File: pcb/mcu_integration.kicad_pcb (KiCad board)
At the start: 4 copper layers, 100 x 100 mm, 104 parts, among them IC1 TL7660IDGKR, IC10 AD844_OPAMP_MEL, IC2 TL081IDT, IC3 FOD814_OPTO_NOSHD, IC4 UA78M33CDCYG3, IC5 FOD814_OPTO_MEL, IC6 AD844_OPAMP_AL, IC7 FOD814_OPTO_AL, IC8 AD844_OPAMP_NOSHD, J1 Micro_SD_Card, J2 M22-6003005, J3 Conn_01x06, U1 STM32F103RBTx, U2 REF192_NOSHD, U3 REF192_AL, U4 REF192_MEL, U5 TPS2069CDBVR_MOSFET, Y1 ECS-80-18-5PX-GM-TR

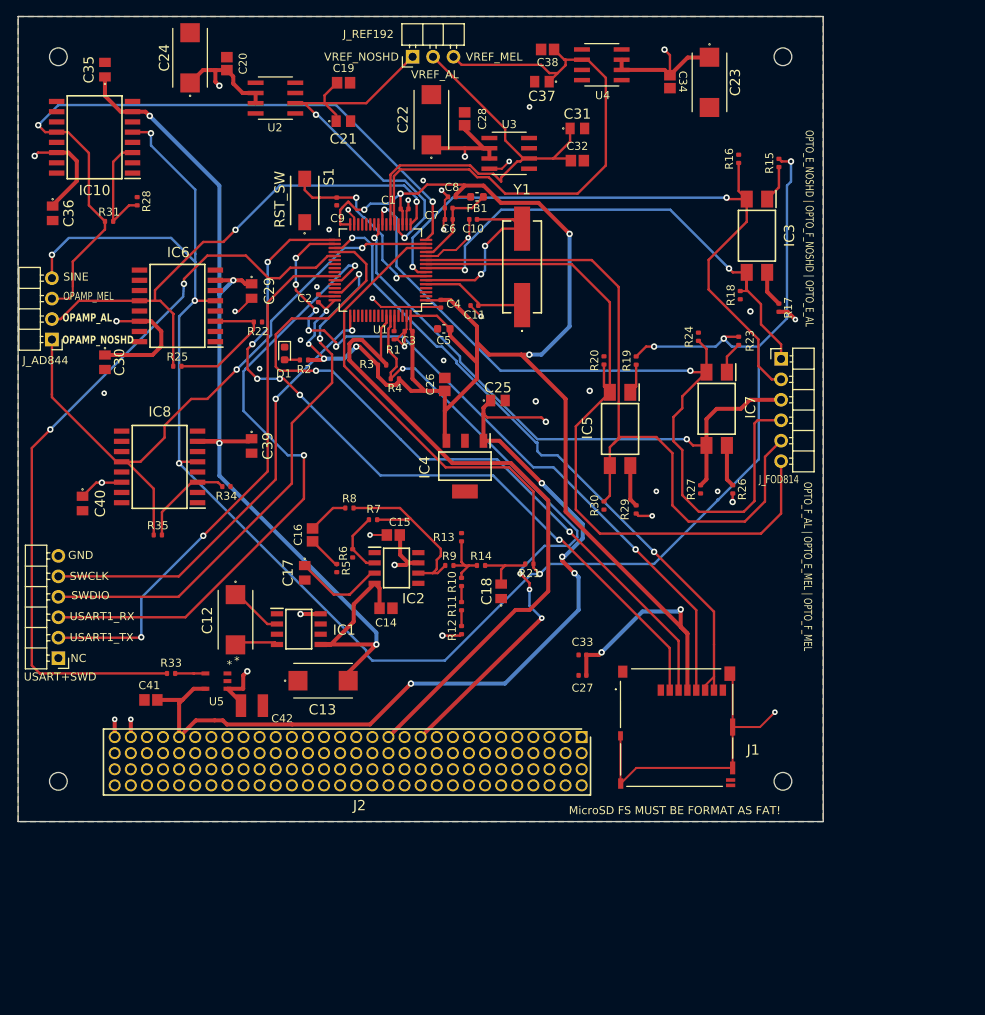
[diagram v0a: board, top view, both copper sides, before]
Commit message: done layout/ratsnet
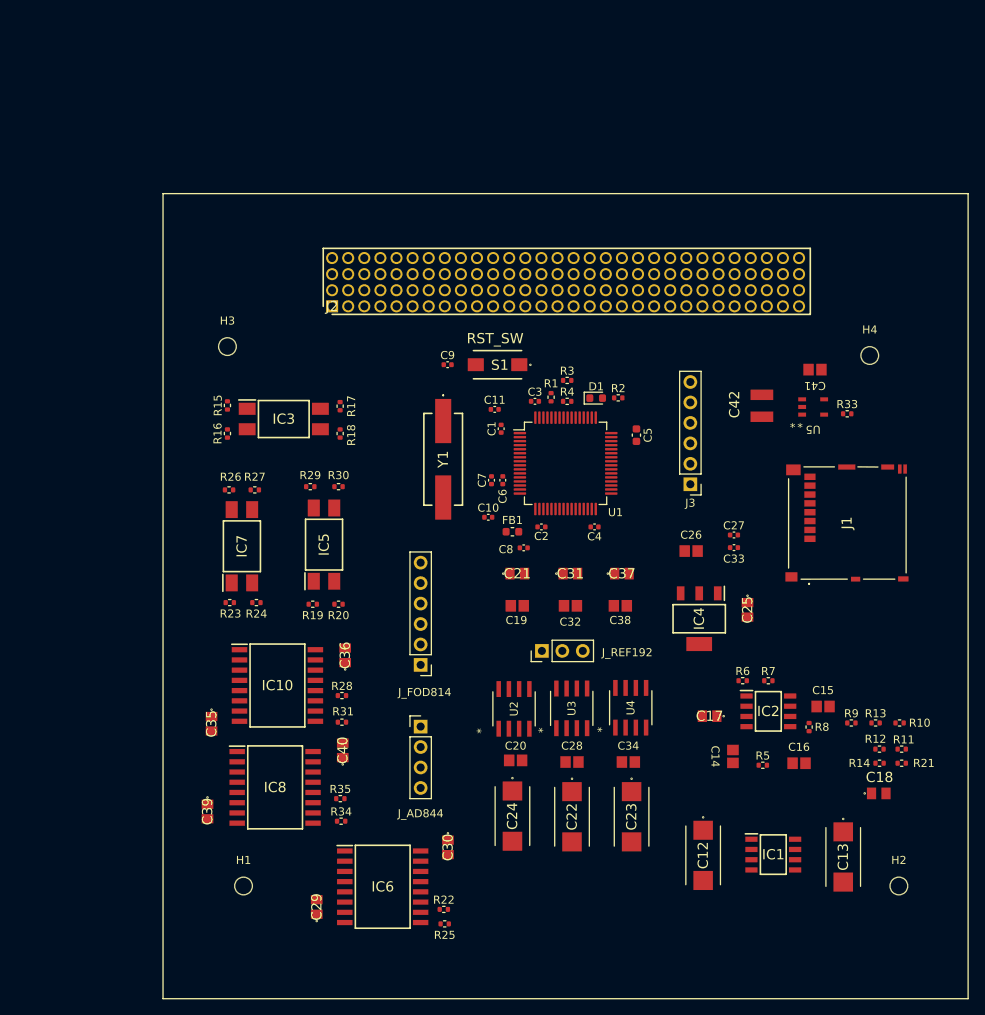
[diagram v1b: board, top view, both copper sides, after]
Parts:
- J3, J_FOD814: footprint Connector_PinHeader_2.54mm:PinHeader_1x06_P2.54mm_Horizontal -> Connector_PinHeader_2.54mm:PinHeader_1x06_P2.54mm_Vertical
- J_AD844: footprint Connector_PinHeader_2.54mm:PinHeader_1x04_P2.54mm_Horizontal -> Connector_PinHeader_2.54mm:PinHeader_1x04_P2.54mm_Vertical
- J_REF192: footprint Connector_PinHeader_2.54mm:PinHeader_1x03_P2.54mm_Horizontal -> Connector_PinHeader_2.54mm:PinHeader_1x03_P2.54mm_Vertical
- moved C24 102.3 mm to (126.4, 134.3), turned to -90 degrees
- moved C20 93.7 mm to (126.8, 127.4), turned to 0 degrees
- moved C41 92.1 mm to (164.0, 78.9)
- moved C23 91.7 mm to (141.2, 134.4)
- moved R33 90.0 mm to (168.0, 84.3), turned to 0 degrees
- moved C22 88.3 mm to (133.8, 134.4), turned to -90 degrees
- moved C34 84.7 mm to (140.8, 127.6), turned to 0 degrees
- moved C35 82.3 mm to (89.0, 122.8), turned to -90 degrees
- moved U5 81.6 mm to (163.8, 83.5), turned to 0 degrees
- moved U2 81.4 mm to (126.6, 121.0), turned to 90 degrees
- moved J3 81.4 mm to (148.5, 93.1)
- moved C28 81.0 mm to (133.8, 127.6), turned to 0 degrees
- moved U4 79.9 mm to (141.1, 120.9), turned to 90 degrees
- moved C29 76.9 mm to (102.1, 145.6), turned to 90 degrees
- moved R25 76.8 mm to (118.0, 147.7)
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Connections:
- C42 pad 1: +5V -> MOSFET_OUTPUT
- IC1 pad 8: +5V -> MOSFET_OUTPUT
- IC3 pad 3: GND -> ADC1_IN11_OPTO_E_NOSHD
- J1 pad 6: /SPI2_MISO -> GND
- J_FOD814 pad 1: GND -> ADC1_IN11_OPTO_E_NOSHD
- R18 pad 2: GND -> ADC1_IN11_OPTO_E_NOSHD
- U1 pad 9: GND -> ADC1_IN11_OPTO_E_NOSHD
- U5 pad 1: +5V -> MOSFET_OUTPUT
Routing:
- net ADC1_IN0_SINE: track 286.5 -> 0.00 mm, vias 8 -> 0
- net +5V: track 240.4 -> 0.00 mm, vias 18 -> 0
- net 3.3V Output: track 218.9 -> 0.00 mm, vias 10 -> 0
- net GND: track 189.4 -> 0.00 mm, vias 29 -> 0
- net -5V Output: track 129.9 -> 0.00 mm, vias 4 -> 0
- net ADC1_IN14_OPTO_F_AL: track 99.1 -> 0.00 mm, vias 2 -> 0
- net /SPI2_CS_NSS: track 95.8 -> 0.00 mm, vias 6 -> 0
- net MOSFET_CONTROL: track 95.3 -> 0.00 mm, vias 2 -> 0
- net /SPI2_MOSI: track 94.9 -> 0.00 mm, vias 2 -> 0
- net ADC1_IN2_OPAMP_MEL: track 90.7 -> 0.00 mm, vias 2 -> 0
- net ADC1_IN12_OPTO_F_MEL: track 90.3 -> 0.00 mm
- net /SPI2_SCK: track 89.8 -> 0.00 mm, vias 6 -> 0
- net ADC1_IN13_OPTO_E_MEL: track 89.4 -> 0.00 mm
- net OBC_I2C_SCL: track 85.4 -> 0.00 mm
- net ADC1_IN10_OPTO_F_NOSHD: track 82.9 -> 0.00 mm, vias 2 -> 0
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- removed copper zone on In2.Cu, net +5V
- removed copper zone on B.Cu, net GND
- removed copper zone on F.Cu, net GND
- removed copper zone on In1.Cu, net GND
- removed copper zone on In2.Cu, net GND
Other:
- board outline removed
